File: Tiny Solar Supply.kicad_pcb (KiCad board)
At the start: 2 copper layers, 41.9 x 18.9 mm, 16 parts, among them J1 Conn_01x02_Pin, J2 Conn_01x02_Pin, J3 Conn_01x02_Pin, J4 Conn_01x02_Pin, Q1 2N7002, U1 AP3015AKTR-G1

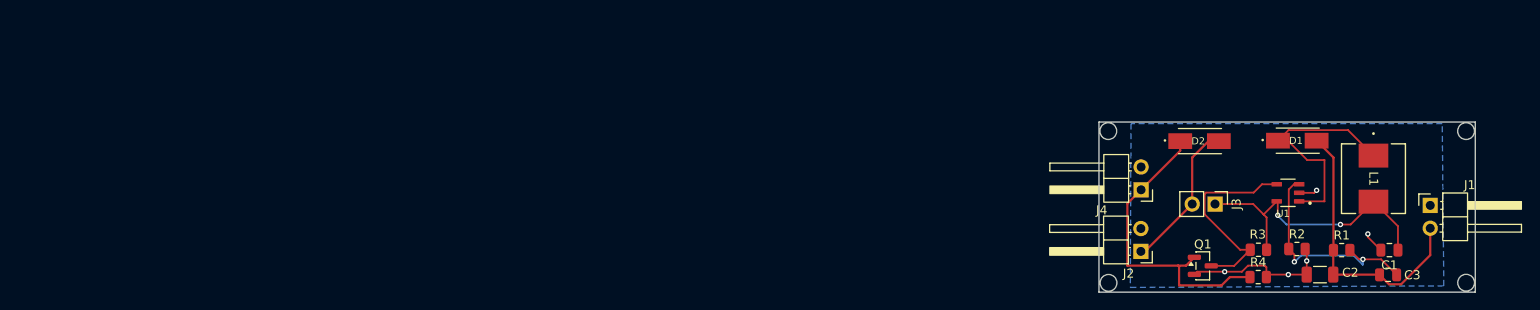
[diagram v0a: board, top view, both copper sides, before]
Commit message: SilkScreen added and project completion
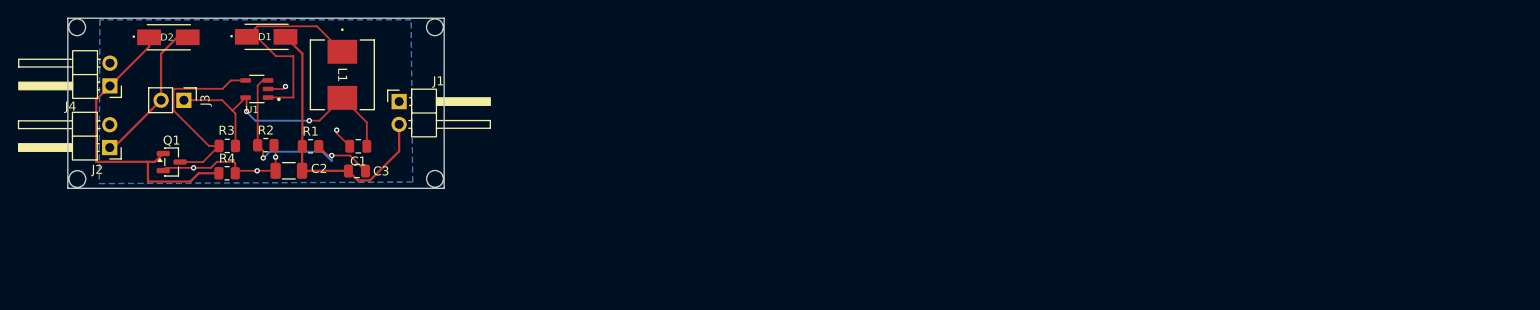
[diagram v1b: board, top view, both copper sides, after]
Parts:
- moved C1 115.3 mm to (96.1, 105.3)
- moved C3 115.3 mm to (95.9, 108.1)
- moved D1 115.3 mm to (85.7, 93.2)
- moved D2 115.3 mm to (74.8, 93.2)
- moved J1 115.3 mm to (100.6, 100.4)
- moved J2 115.3 mm to (68.4, 105.5)
- moved J3 115.3 mm to (76.7, 100.2)
- moved J4 115.3 mm to (68.5, 98.6)
- moved L1 115.3 mm to (94.3, 97.4)
- moved R1 115.3 mm to (90.8, 105.3)
- moved C2 115.3 mm to (88.4, 108.1)
- moved Q1 115.3 mm to (75.3, 107.1)
- moved R2 115.3 mm to (85.8, 105.2)
- moved R3 115.3 mm to (81.5, 105.3)
- moved R4 115.3 mm to (81.5, 108.3)
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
